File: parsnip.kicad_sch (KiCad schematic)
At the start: 18 parts, among them J1 I2C1, J2 SPI BUS, J7 I2C2, U7 ESP32-S3-WROOM-1

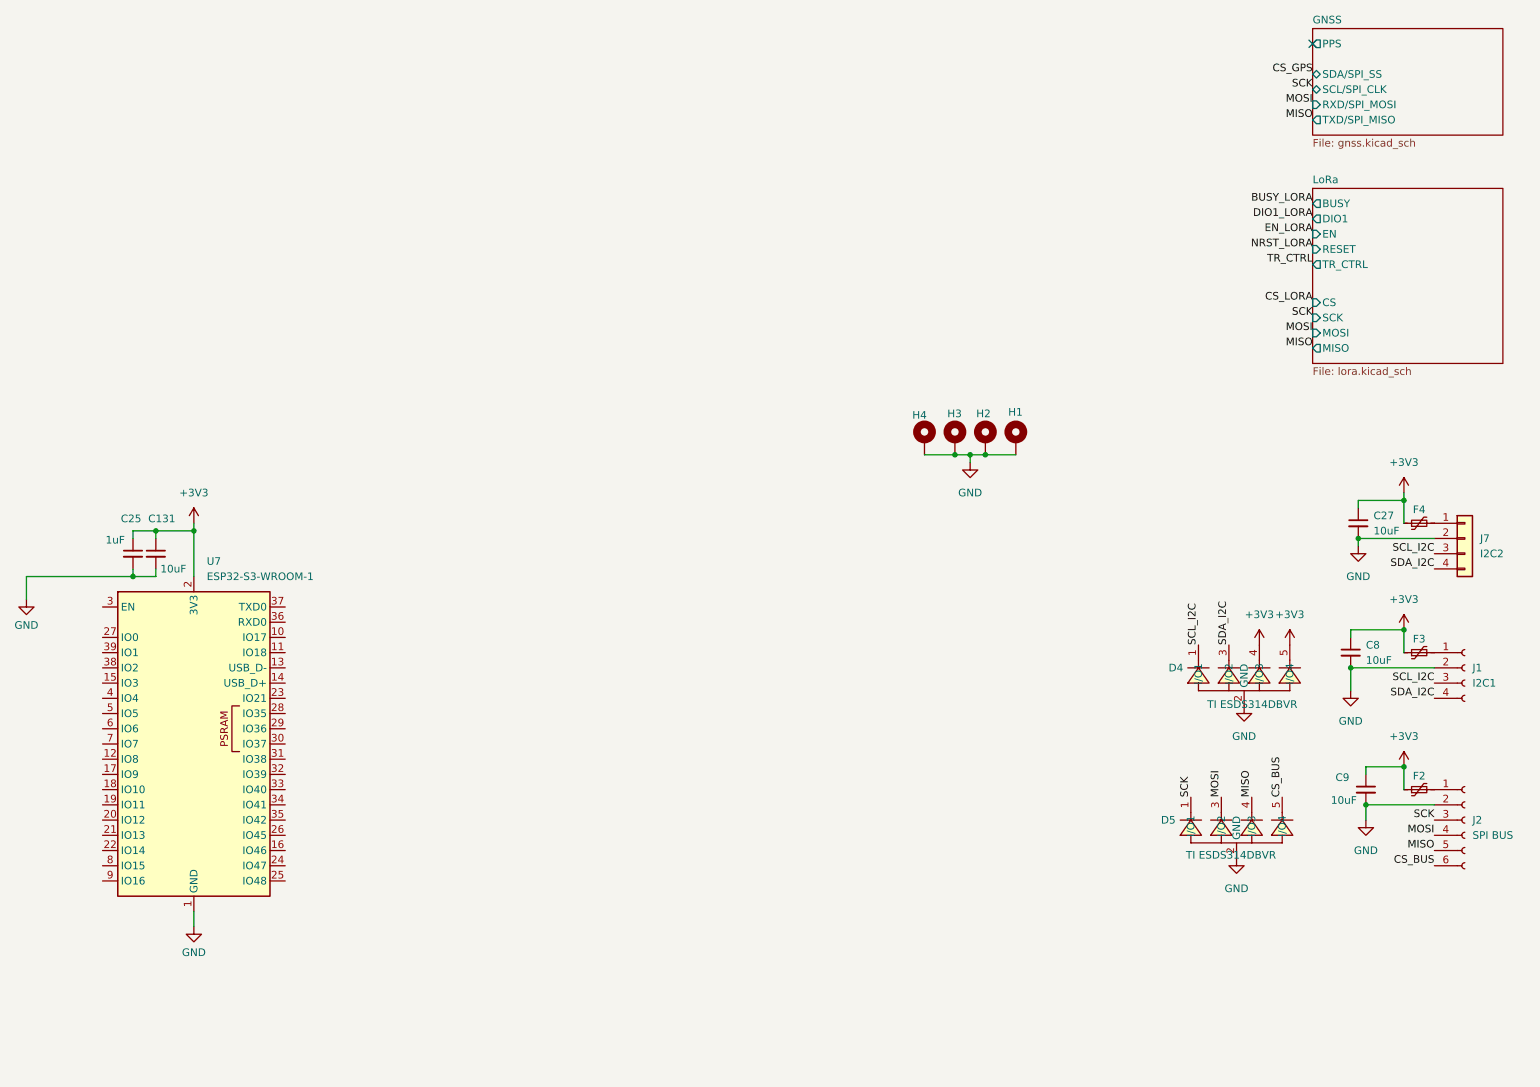
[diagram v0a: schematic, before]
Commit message: usb-org
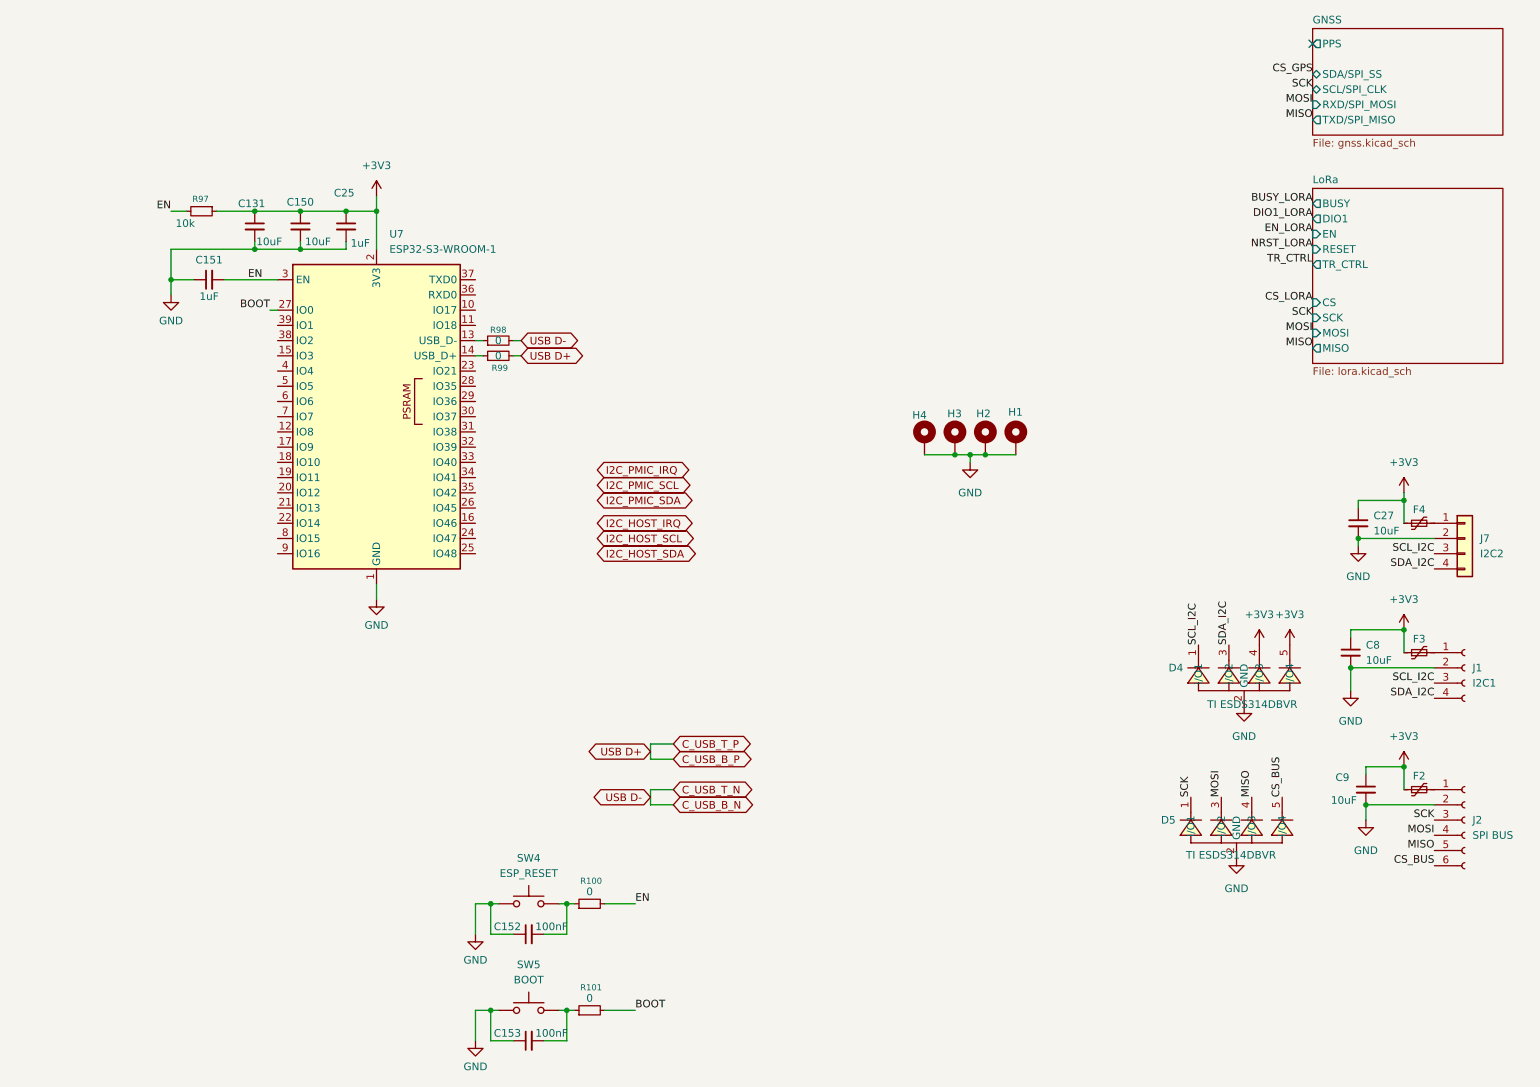
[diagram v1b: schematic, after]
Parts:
- added C150: 10uF, symbol Device:C_Small
- added C151: 1uF, symbol Device:C_Small
- added C152, C153: 100nF, Capacitor_SMD:C_0402_1005Metric, symbol Device:C_Small
- added R100, R101, R98, R99: 0, Resistor_SMD:R_0402_1005Metric, symbol Device:R_Small
- added R97: 10k, symbol Device:R_Small
- added SW4: ESP_RESET, symbol Switch:SW_Push
- added SW5: BOOT, symbol Switch:SW_Push
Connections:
- net +3V3: now also C150.1, R97.1
- net GND: now also C150.2, C151.1, C152.1, C153.1, SW4.1, SW5.1
- net at U7.13 (USB_D-): now also R98.1
- net at U7.14 (USB_D+): now also R99.1
- net BOOT: now reaches U7.27 (IO0)
- net BOOT: now also R101.2
- net EN: now reaches U7.3 (EN)
- net EN: now also C151.2, R100.2, R97.2
- new net: C153.2, R101.1, SW5.2
- new net: C152.2, R100.1, SW4.2
- new net C_USB_B_N: R98.2
- new net C_USB_B_P: R99.2
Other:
- moved on the sheet: C131, C25, U7
